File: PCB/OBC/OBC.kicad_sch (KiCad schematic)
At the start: 5 parts, among them J1 Conn_02x24_Odd_Even

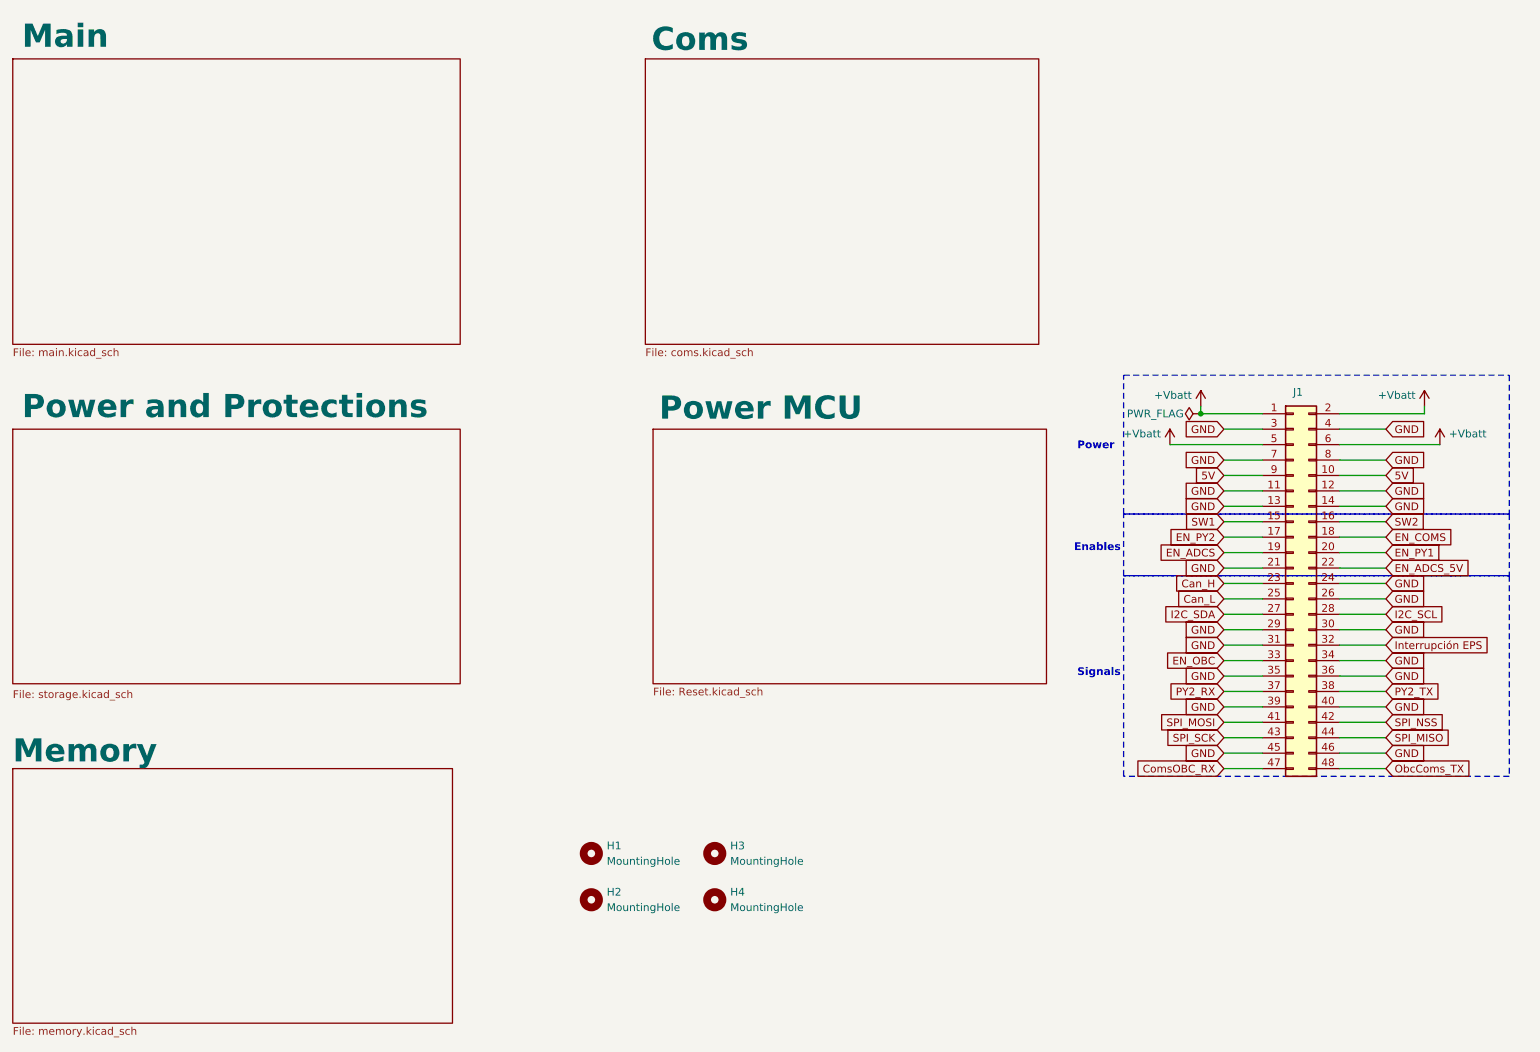
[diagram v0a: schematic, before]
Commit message: Finishing schematics
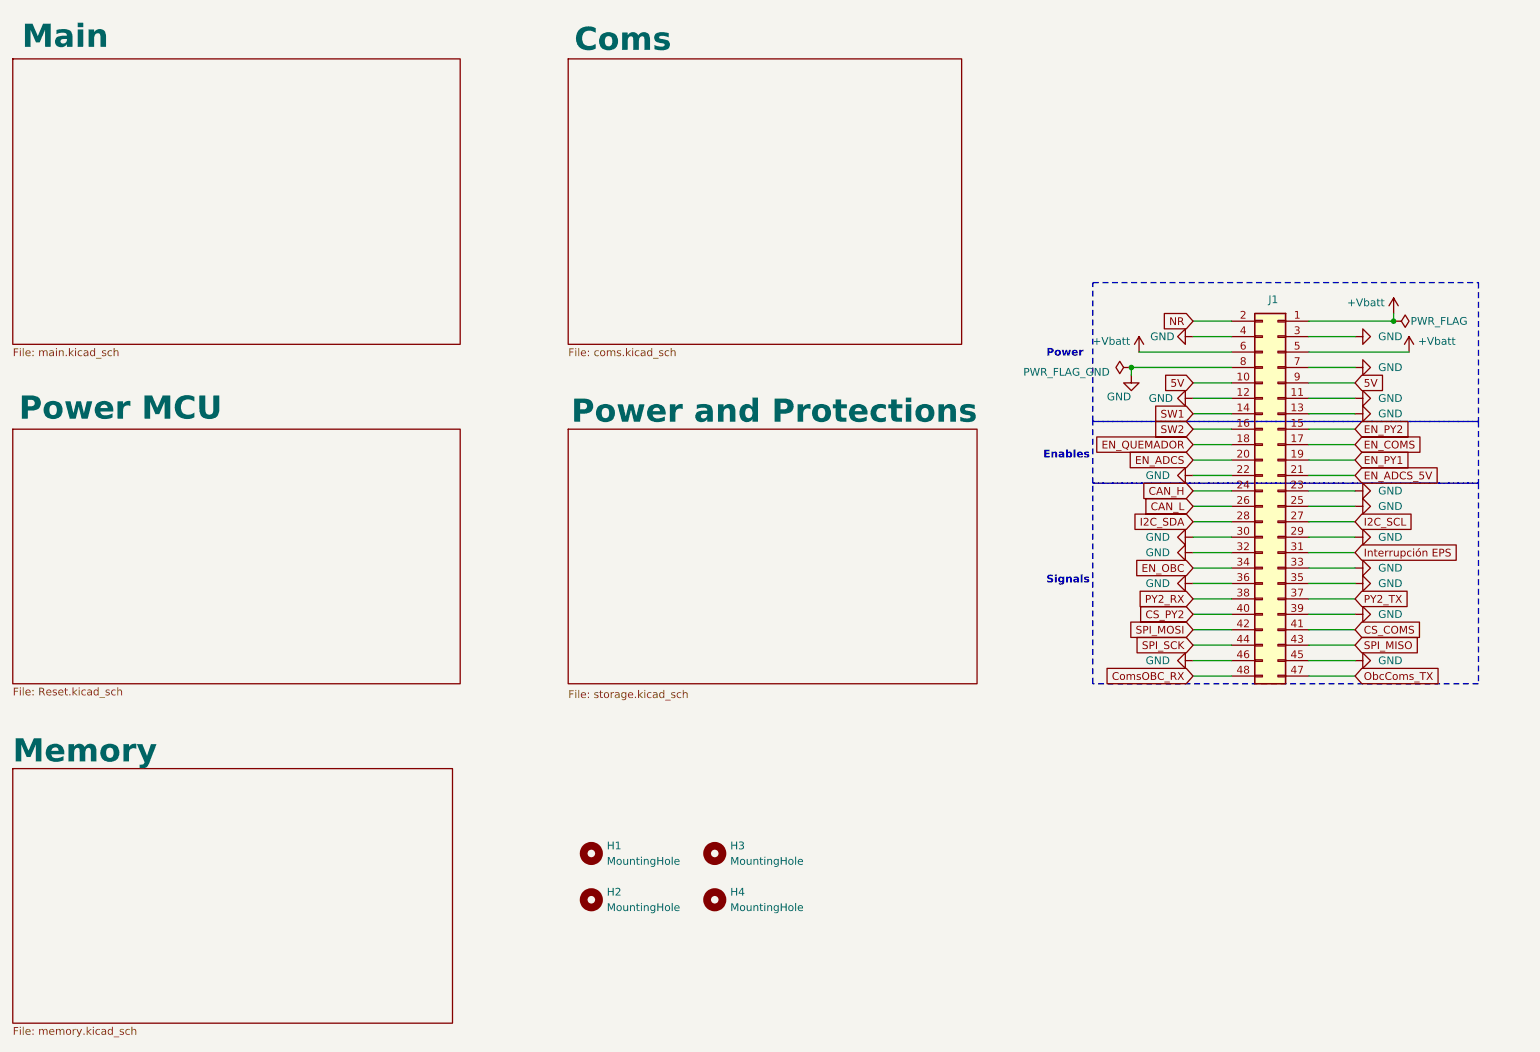
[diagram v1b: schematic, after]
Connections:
- net Can_H is gone; now on net GND: J1.23 (Pin_23)
- net Can_L is gone; now on net GND: J1.25 (Pin_25)
- net SPI_NSS is gone; now on net SPI_MOSI: J1.42 (Pin_42)
- net +Vbatt: no longer J1.2 (Pin_2)
- net ComsOBC_RX: now also J1.48 (Pin_48); no longer J1.47 (Pin_47)
- net EN_ADCS: now also J1.20 (Pin_20); no longer J1.19 (Pin_19)
- net EN_ADCS_5V: now also J1.21 (Pin_21); no longer J1.22 (Pin_22)
- net EN_COMS: now also J1.17 (Pin_17); no longer J1.18 (Pin_18)
- net EN_OBC: now also J1.34 (Pin_34); no longer J1.33 (Pin_33)
- net EN_PY1: now also J1.19 (Pin_19); no longer J1.20 (Pin_20)
- net EN_PY2: now also J1.15 (Pin_15); no longer J1.17 (Pin_17)
- net GND: now also J1.22 (Pin_22), J1.32 (Pin_32), J1.33 (Pin_33); no longer J1.14 (Pin_14), J1.21 (Pin_21), J1.24 (Pin_24), J1.26 (Pin_26), J1.31 (Pin_31), J1.34 (Pin_34), J1.40 (Pin_40)
- net I2C_SCL: now also J1.27 (Pin_27); no longer J1.28 (Pin_28)
- net I2C_SDA: now also J1.28 (Pin_28); no longer J1.27 (Pin_27)
- net Interrupción EPS: now also J1.31 (Pin_31); no longer J1.32 (Pin_32)
- net ObcComs_TX: now also J1.47 (Pin_47); no longer J1.48 (Pin_48)
- net PY2_RX: now also J1.38 (Pin_38); no longer J1.37 (Pin_37)
- net PY2_TX: now also J1.37 (Pin_37); no longer J1.38 (Pin_38)
- net SPI_MISO: now also J1.43 (Pin_43); no longer J1.44 (Pin_44)
- net SPI_MOSI: no longer J1.41 (Pin_41)
- net SPI_SCK: now also J1.44 (Pin_44); no longer J1.43 (Pin_43)
- net SW1: now also J1.14 (Pin_14); no longer J1.15 (Pin_15)
- new net CAN_H: J1.24 (Pin_24)
- new net CAN_L: J1.26 (Pin_26)
- new net CS_COMS: J1.41 (Pin_41)
- new net CS_PY2: J1.40 (Pin_40)
- new net EN_QUEMADOR: J1.18 (Pin_18)
- new net NR: J1.2 (Pin_2)
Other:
- moved on the sheet: J1

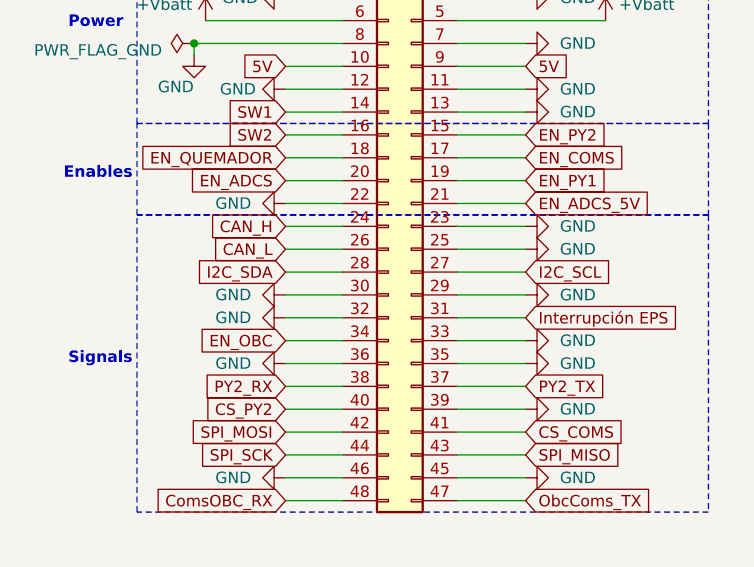
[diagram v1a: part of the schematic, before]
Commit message: PC104
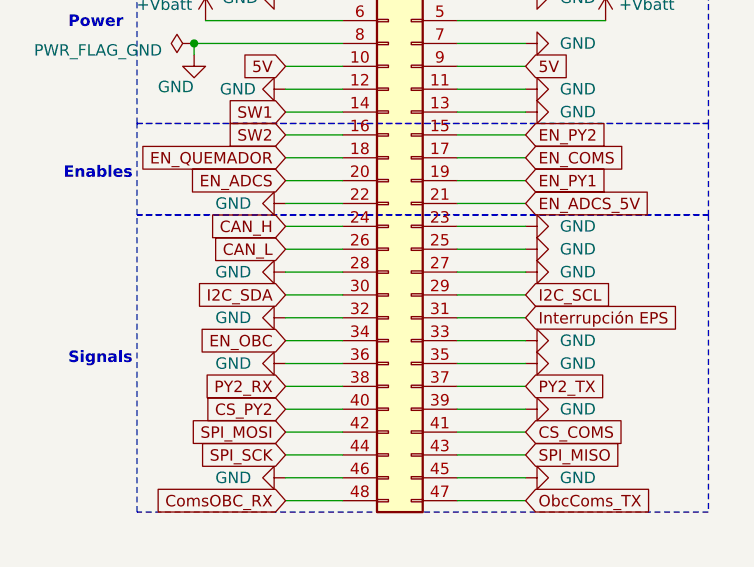
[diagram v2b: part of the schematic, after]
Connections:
- net GND: now also J1.27 (Pin_27), J1.28 (Pin_28); no longer J1.29 (Pin_29), J1.30 (Pin_30)
- net I2C_SCL: now also J1.29 (Pin_29); no longer J1.27 (Pin_27)
- net I2C_SDA: now also J1.30 (Pin_30); no longer J1.28 (Pin_28)

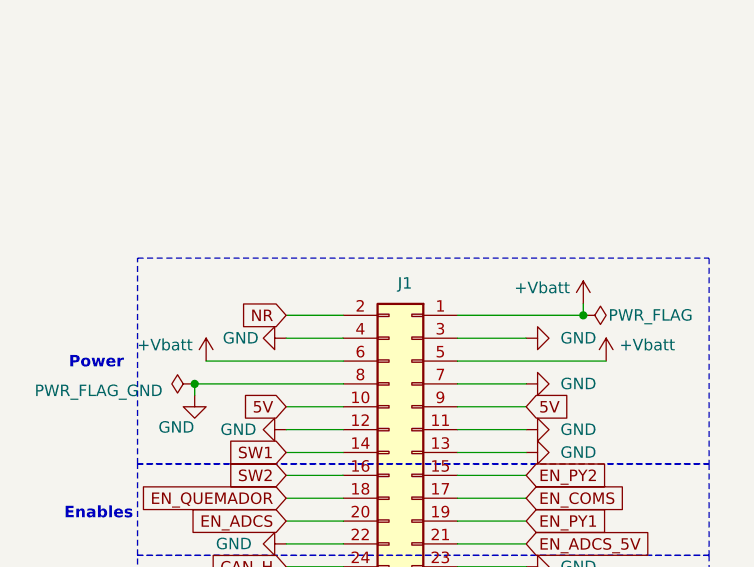
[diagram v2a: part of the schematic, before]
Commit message: Coms memory finished
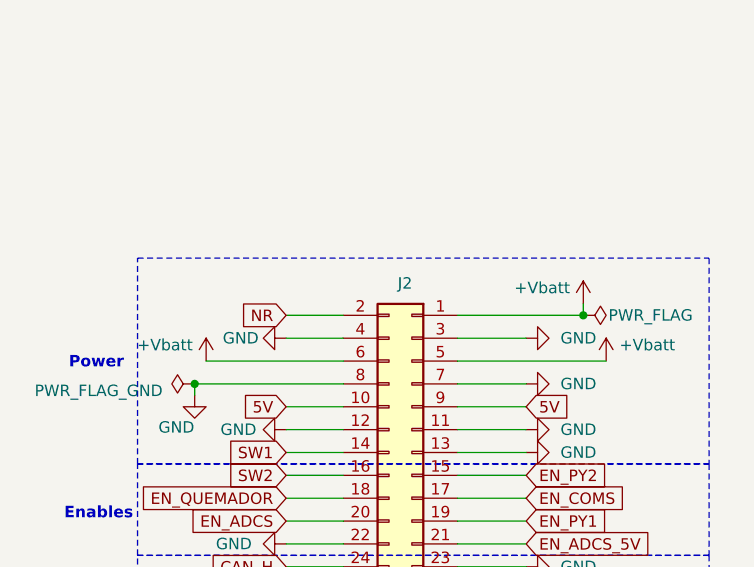
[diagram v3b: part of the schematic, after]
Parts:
- renumbered J1 to J2
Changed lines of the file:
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@@
 		(on_board yes)
 		(dnp no)
-		(property "Reference" "J1"
+		(property "Reference" "J2"
 			(at 240.538 66.294 0)
 			(effects
@@
 			(project "OBC"
 				(path "/e2c03eef-3b12-44a7-ba52-633d5337a24a"
-					(reference "J1")
+					(reference "J2")
 					(unit 1)
 				)
